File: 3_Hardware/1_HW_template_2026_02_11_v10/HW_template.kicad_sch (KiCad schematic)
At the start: 5 parts, among them P1 ${SIM.PARAMS}, P2 ${SIM.PARAMS}

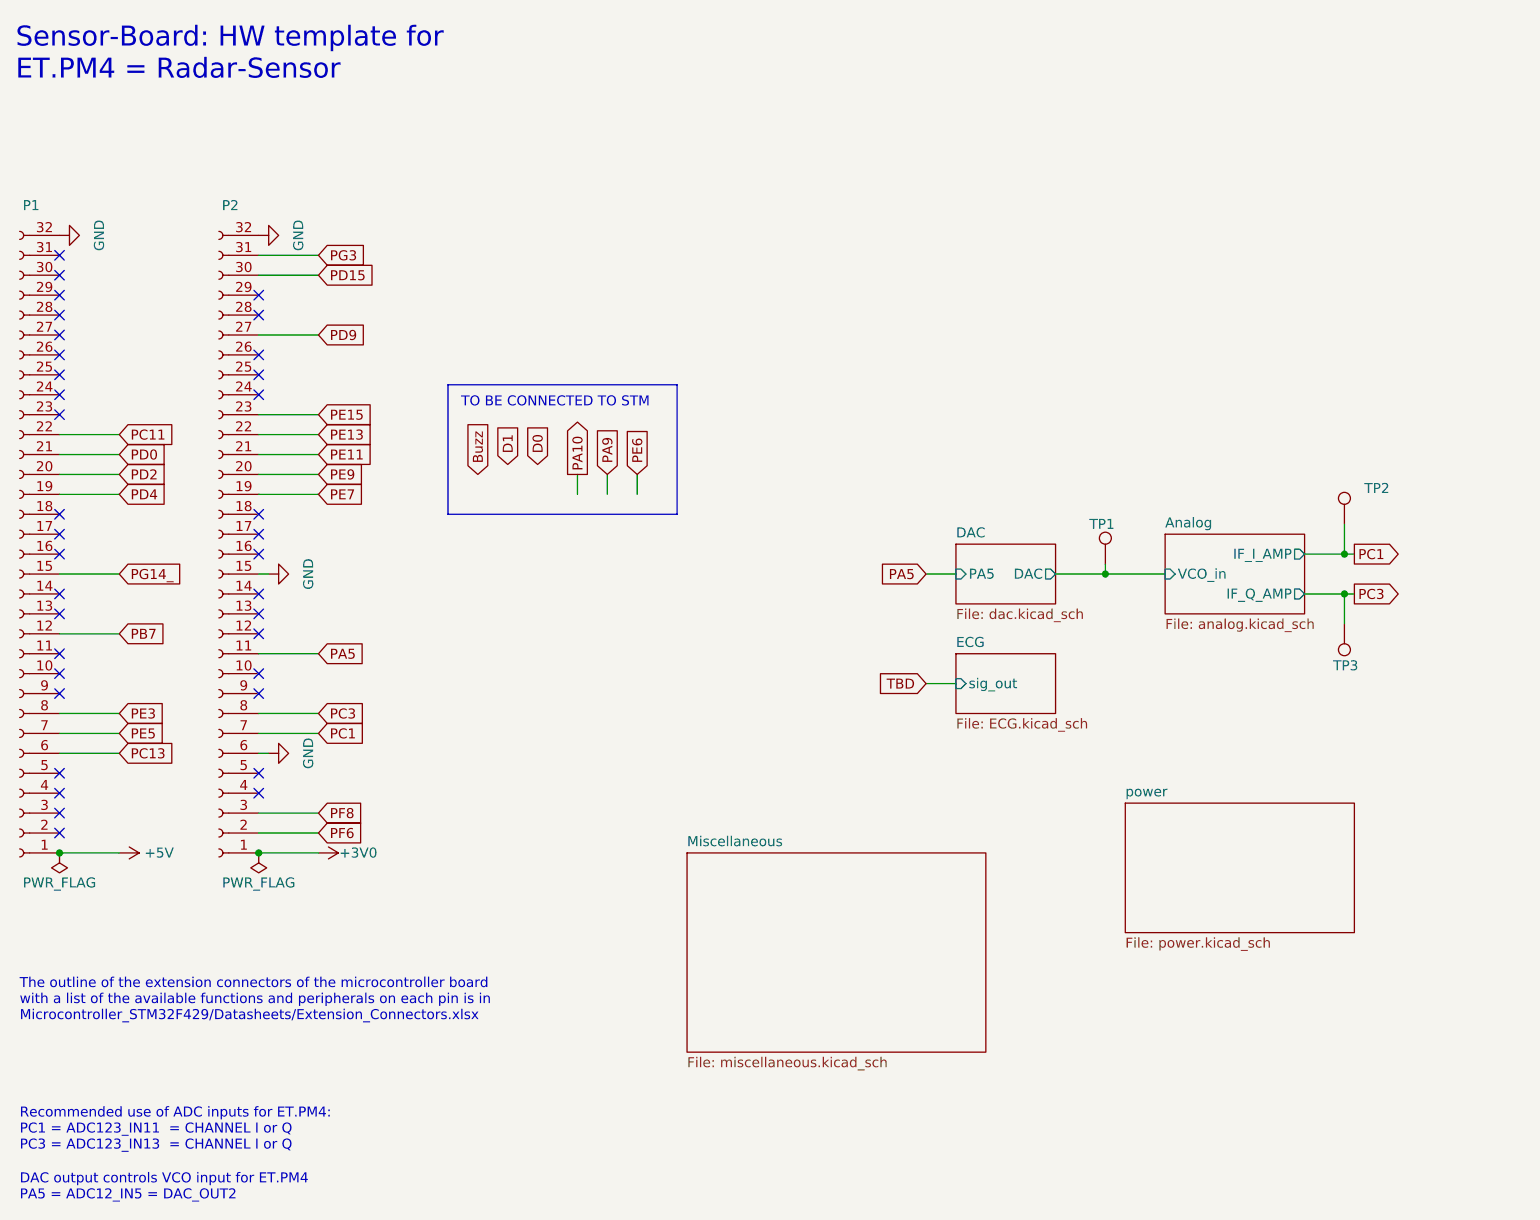
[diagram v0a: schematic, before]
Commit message: pcb schematics finished + layout
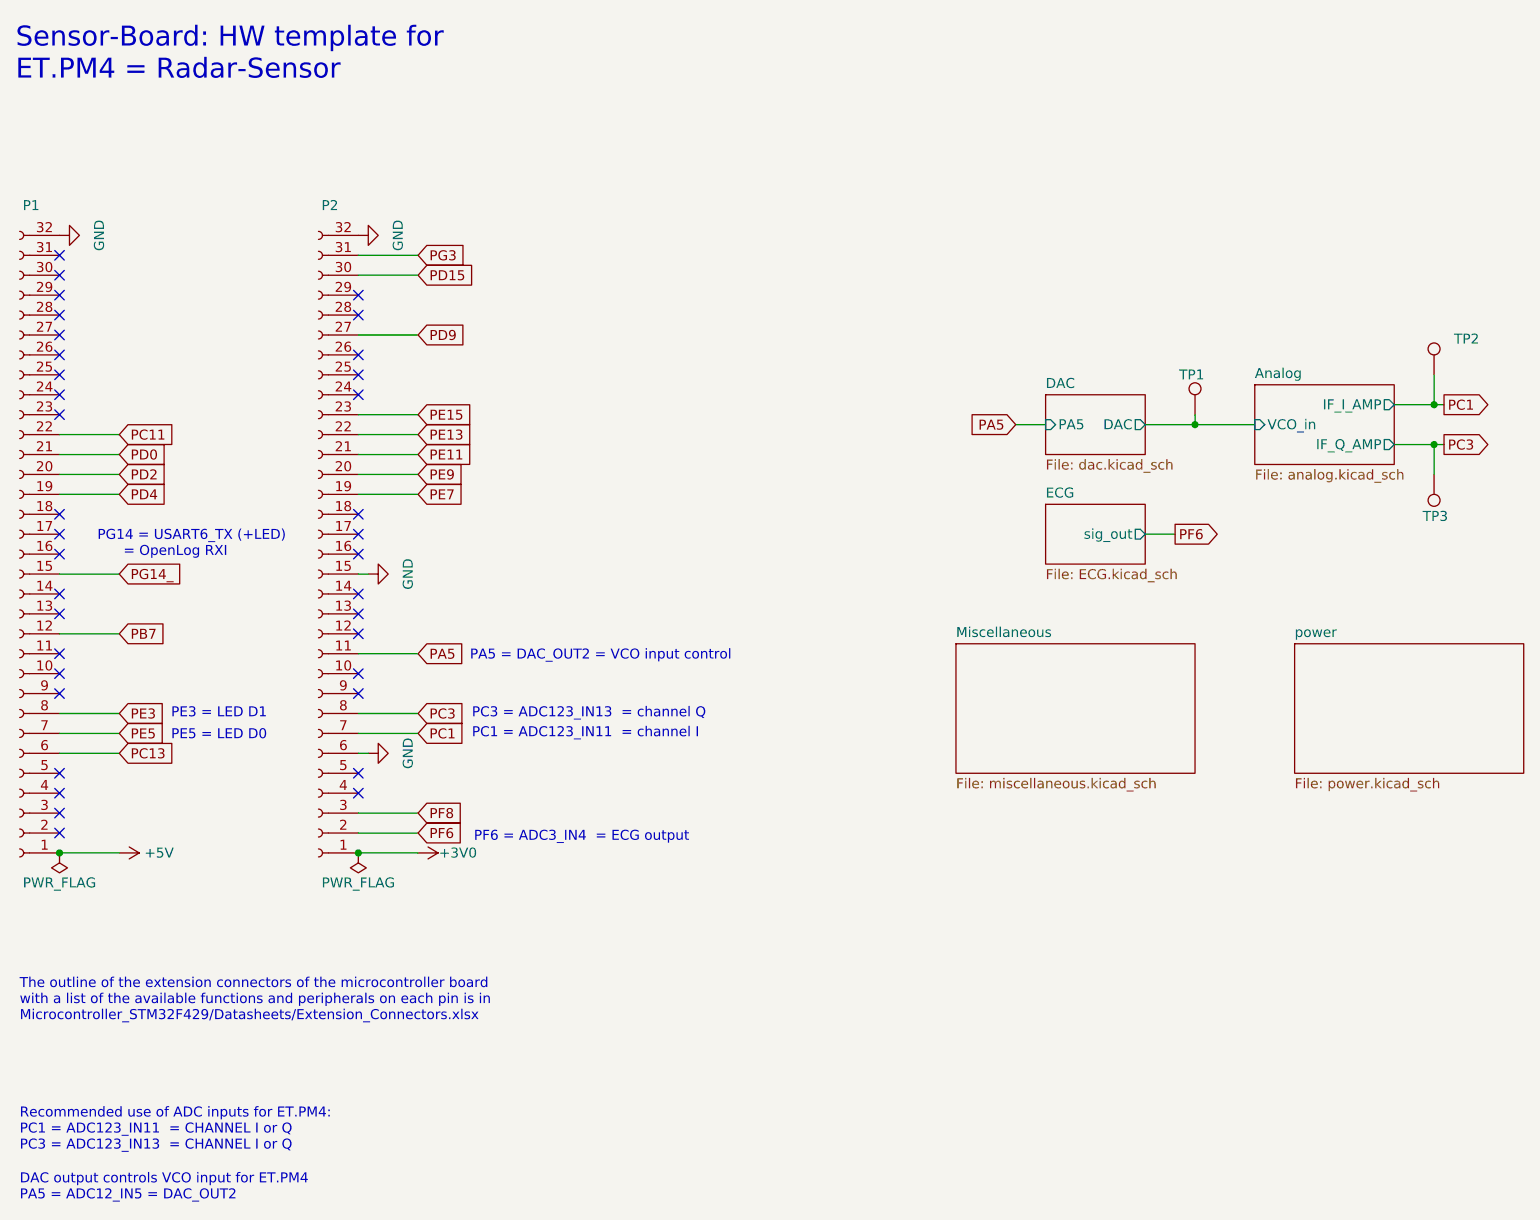
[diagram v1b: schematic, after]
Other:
- note added: "PA5 = DAC_OUT2 = VCO input control"
- note added: "PC1 = ADC123_IN11 = channel I"
- note added: "PC3 = ADC123_IN13 = channel Q"
- note added: "PE3 = LED D1"
- note added: "PE5 = LED D0"
- note added: "PF6 = ADC3_IN4 = ECG output"
- note added: "PG14 = USART6_TX (+LED) = OpenLog RXI"
- note removed: "TO BE CONNECTED TO STM"
- moved on the sheet: P2, TP1, TP2, TP3
